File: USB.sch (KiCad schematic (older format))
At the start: 2 parts, among them U3 TPD4S012DRYR, U4 USB_Micro_B

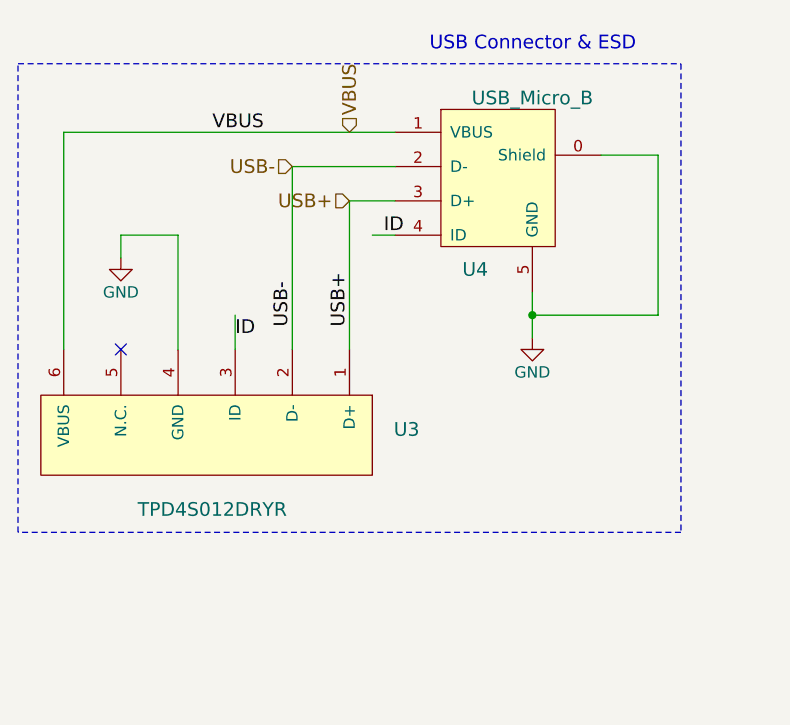
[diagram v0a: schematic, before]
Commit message: Updated to Rev2.0
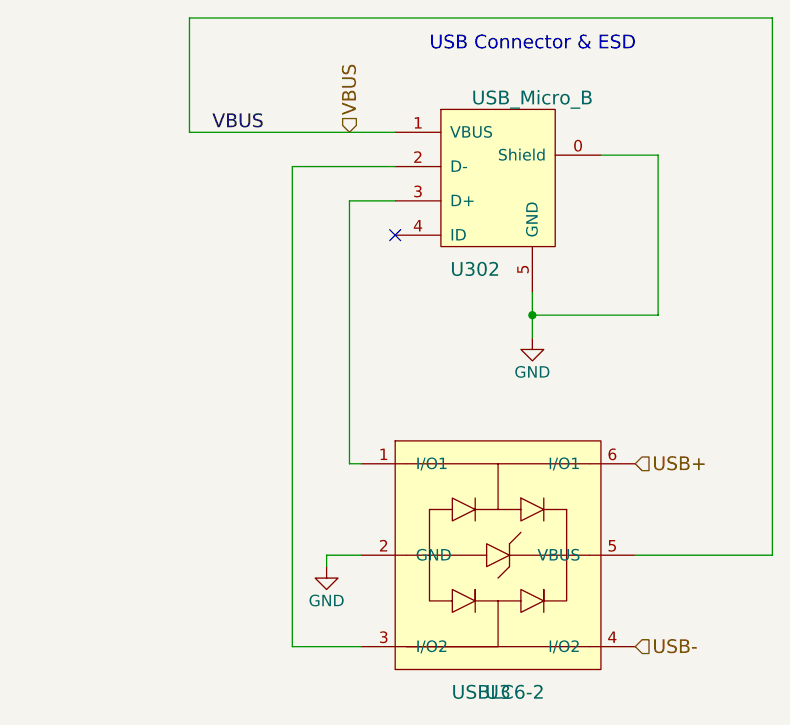
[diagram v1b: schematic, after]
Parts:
- removed U3: TPD4S012DRYR, Footprints:TPD4S012DRYR, symbol TPD4S012DRYR
- added U3: USBLC6-2, TO_SOT_Packages_SMD:SOT-23-6_Handsoldering, symbol USBLC6-2
- renumbered U4 to U302
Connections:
- net labels removed: ID
- wire segments 15 -> 17
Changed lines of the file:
@@
 EESchema Schematic File Version 2
+LIBS:NEOM_0-rescue
 LIBS:power
 LIBS:device
@@
 LIBS:contrib
 LIBS:valves
-LIBS:stm32f070f6p6
 LIBS:tpd4s012dryr
 LIBS:lm3940
 LIBS:tactile_button
+LIBS:NEOM_0
 LIBS:NEOM_0-cache
 EELAYER 25 0
@@
 $Descr A4 11693 8268
 encoding utf-8
-Sheet 3 4
+Sheet 3 5
 Title ""
 Date ""
@@
 Comment4 ""
 $EndDescr
-$Comp
-L TPD4S012DRYR U3
-U 1 1 5A19F702
-P 3950 4900
-F 0 "U3" V 3350 7150 60  0000 C CNN
-F 1 "TPD4S012DRYR" V 3700 6300 60  0000 C CNN
-F 2 "Footprints:TPD4S012DRYR" H 3950 4900 60  0001 C CNN
-F 3 "http://www.ti.com/lit/ds/symlink/tpd4s012.pdf" H 3950 4900 60  0001 C CNN
-F 4 "296-24244-1-ND" V 3950 4900 60  0001 C CNN "DigiKeyPartNumber	"
-F 5 "TPD4S012DRYR" V 3950 4900 60  0001 C CNN "ManufacturerPartNumber	"
-	1    3950 4900
-	0    1    1    0
-$EndComp
-NoConn ~ 4950 3950
+NoConn ~ 6150 3450
 $Comp
 L GND #PWR011
@@
 L GND #PWR012
 U 1 1 5A19F710
-P 4950 3550
-F 0 "#PWR012" H 4950 3300 50  0001 C CNN
-F 1 "GND" H 4950 3400 50  0000 C CNN
-F 2 "" H 4950 3550 50  0000 C CNN
-F 3 "" H 4950 3550 50  0000 C CNN
-	1    4950 3550
+P 5850 4900
+F 0 "#PWR012" H 5850 4650 50  0001 C CNN
+F 1 "GND" H 5850 4750 50  0000 C CNN
+F 2 "" H 5850 4900 50  0000 C CNN
+F 3 "" H 5850 4900 50  0000 C CNN
+	1    5850 4900
 	1    0    0    -1
 $EndComp
-Wire Wire Line
-	4950 3550 4950 3450
-Wire Wire Line
-	4950 3450 5200 3450
-Wire Wire Line
-	5200 3450 5200 3950
-$Comp
-L USB_Micro_B U4
-U 1 1 5A19F71B
-P 6350 3650
-F 0 "U4" H 6500 3700 60  0000 C CNN
-F 1 "USB_Micro_B" H 6750 4450 60  0000 C CNN
-F 2 "Footprints2:MICRO_USB_B_Type" H 6350 3650 60  0001 C CNN
-F 3 "http://cdn.amphenol-icc.com/media/wysiwyg/files/drawing/10118192.pdf" H 6350 3650 60  0001 C CNN
-F 4 "609-4613-1-ND" H 6350 3650 60  0001 C CNN "DigiKeyPartNumber	"
-F 5 "10118192-0001LF" H 6350 3650 60  0001 C CNN "ManufacturerPartNumber	"
-	1    6350 3650
-	1    0    0    -1
-$EndComp
-Wire Wire Line
-	4700 3000 6150 3000
-Wire Wire Line
-	4700 3000 4700 3950
 Wire Wire Line
 	5700 3150 6150 3150
@@
 	6150 3300 5950 3300
 Wire Wire Line
-	5950 3300 5950 3950
-Text Label 6100 3450 0    60   ~ 0
-ID
-Text Label 5450 3900 0    60   ~ 0
-ID
+	5950 3300 5950 4450
 Wire Wire Line
 	6750 3700 6750 3900
@@
 Text Label 5350 3000 0    60   ~ 0
 VBUS
-Wire Wire Line
-	6150 3450 6050 3450
-Wire Wire Line
-	5450 3950 5450 3800
-Wire Notes Line
-	4500 2700 7400 2700
-Wire Notes Line
-	7400 2700 7400 4750
-Wire Notes Line
-	7400 4750 4500 4750
-Wire Notes Line
-	4500 4750 4500 2700
 Text Notes 6300 2650 0    60   ~ 0
 USB Connector & ESD
 Wire Wire Line
-	5700 3150 5700 3950
-Text Label 5950 3850 1    60   ~ 0
-USB+
-Text Label 5700 3850 1    60   ~ 0
+	5700 3150 5700 5250
+Text HLabel 7200 5250 2    60   Input ~ 0
 USB-
-Text HLabel 5700 3150 0    60   Input ~ 0
-USB-
-Text HLabel 5950 3300 0    60   Input ~ 0
+Text HLabel 7200 4450 2    60   Input ~ 0
 USB+
 Text HLabel 5950 3000 1    60   Input ~ 0
 VBUS
+$Comp
+L USBLC6-2 U3
+U 1 1 5A37C531
+P 6600 5450
+F 0 "U3" H 6600 5450 60  0000 C CNN
+F 1 "USBLC6-2" H 6600 5450 60  0000 C CNN
+F 2 "TO_SOT_Packages_SMD:SOT-23-6_Handsoldering" H 6600 5450 60  0001 C CNN
+F 3 "" H 6600 5450 60  0001 C CNN
+	1    6600 5450
+	1    0    0    -1
+$EndComp
+Wire Wire Line
+	5950 4450 6000 4450
+Wire Wire Line
+	5700 5250 6000 5250
+Wire Wire Line
+	6150 3000 5250 3000
+Wire Wire Line
+	5250 3000 5250 2500
+Wire Wire Line
+	5250 2500 7800 2500
+Wire Wire Line
+	7800 2500 7800 4850
+Wire Wire Line
+	7800 4850 7200 4850
+Wire Wire Line
+	6000 4850 5850 4850
+Wire Wire Line
+	5850 4850 5850 4900
+$Comp
+L USB_Micro_B U302
+U 1 1 5A19F71B
+P 6350 3650
+F 0 "U302" H 6500 3700 60  0000 C CNN
+F 1 "USB_Micro_B" H 6750 4450 60  0000 C CNN
+F 2 "Footprints2:MICRO_USB_B_Type" H 6350 3650 60  0001 C CNN
+F 3 "http://cdn.amphenol-icc.com/media/wysiwyg/files/drawing/10118192.pdf" H 6350 3650 60  0001 C CNN
+F 4 "609-4613-1-ND" H 6350 3650 60  0001 C CNN "DigiKeyPartNumber	"
+F 5 "10118192-0001LF" H 6350 3650 60  0001 C CNN "ManufacturerPartNumber	"
+	1    6350 3650
+	1    0    0    -1
+$EndComp
 $EndSCHEMATC
